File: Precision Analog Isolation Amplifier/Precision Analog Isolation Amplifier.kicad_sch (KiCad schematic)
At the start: 20 parts, among them J1 Conn_Coaxial, J2 Conn_Coaxial, Q1 2N3906, U1 HCNR201, U2 TLV172IDCK, U3 TLV172IDCK

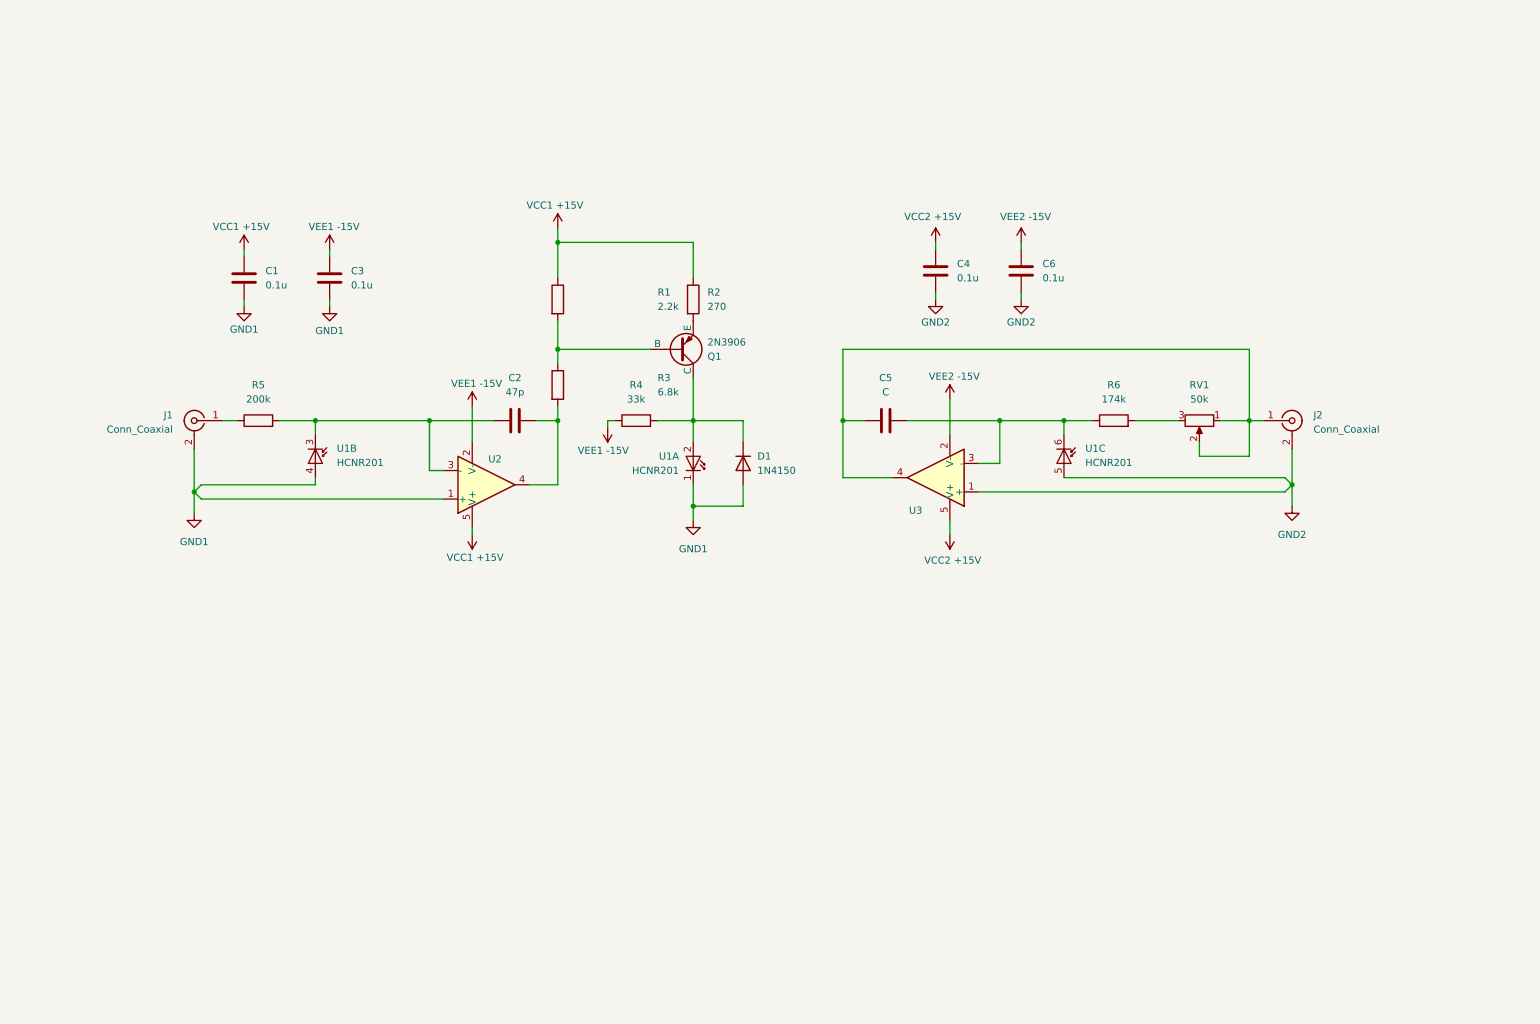
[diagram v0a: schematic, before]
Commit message: Add few components & Start PCB design
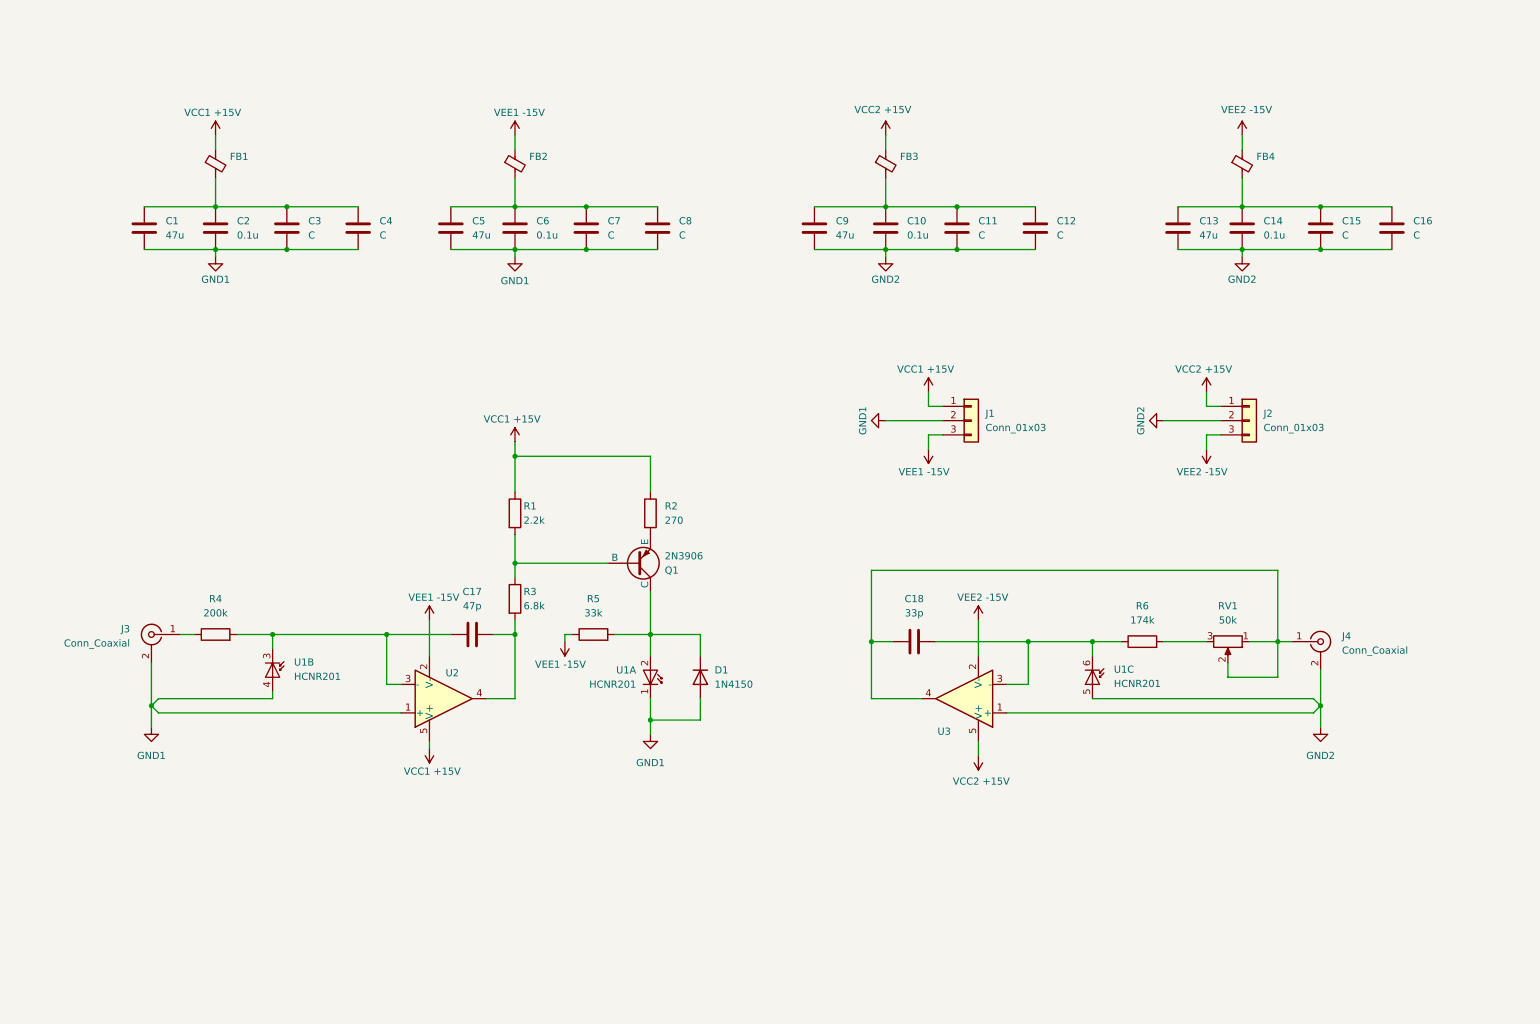
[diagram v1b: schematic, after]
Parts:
- added C1, C13, C5, C9: 47u, Capacitor_SMD:C_0805_2012Metric_Pad1.18x1.45mm_HandSolder, symbol Device:C
- added C11, C12, C15, C16, C3, C4, C7, C8: C, Capacitor_SMD:C_0805_2012Metric_Pad1.18x1.45mm_HandSolder, symbol Device:C
- added FB1, FB2, FB3, FB4: FerriteBead_Small, Inductor_SMD:L_1206_3216Metric, symbol Device:FerriteBead_Small
- added J1, J2: Conn_01x03, Connector_PinHeader_2.54mm:PinHeader_1x03_P2.54mm_Vertical, symbol Connector_Generic:Conn_01x03
- C10: renamed from C4; footprint (none) -> Capacitor_SMD:C_0805_2012Metric_Pad1.18x1.45mm_HandSolder
- C14: renamed from C6; footprint (none) -> Capacitor_SMD:C_0805_2012Metric_Pad1.18x1.45mm_HandSolder
- C17: renamed from C2; footprint (none) -> Capacitor_SMD:C_0805_2012Metric_Pad1.18x1.45mm_HandSolder
- C18: renamed from C5; value C -> 33p; footprint (none) -> Capacitor_SMD:C_0805_2012Metric_Pad1.18x1.45mm_HandSolder
- C2: renamed from C1; footprint (none) -> Capacitor_SMD:C_0805_2012Metric_Pad1.18x1.45mm_HandSolder
- C6: renamed from C3; footprint (none) -> Capacitor_SMD:C_0805_2012Metric_Pad1.18x1.45mm_HandSolder
- J3: renamed from J1; footprint (none) -> Connector_Coaxial:SMA_Amphenol_132289_EdgeMount
- J4: renamed from J2; footprint (none) -> Connector_Coaxial:SMA_Amphenol_132289_EdgeMount
- R1, R2, R3, R6: footprint (none) -> Resistor_SMD:R_0805_2012Metric_Pad1.20x1.40mm_HandSolder
- R4: renamed from R5; footprint (none) -> Resistor_SMD:R_0805_2012Metric_Pad1.20x1.40mm_HandSolder
- R5: renamed from R4; footprint (none) -> Resistor_SMD:R_0805_2012Metric_Pad1.20x1.40mm_HandSolder
- RV1: footprint (none) -> Potentiometer_THT:Potentiometer_Bourns_3386W_Horizontal
- U2, U3: footprint Package_TO_SOT_SMD:SOT-353_SC-70-5 -> (none)
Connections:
- net GND1: now also C1.1, C3.1, C4.1, C5.1, C7.1, C8.1, J1.2 (Pin_2)
- net GND2: now also C11.1, C12.1, C13.1, C15.1, C16.1, C9.1, J2.2 (Pin_2)
- net VCC1 +15V: now also FB1.1, J1.1 (Pin_1); no longer C2.2
- net VCC2 +15V: now also FB3.1, J2.1 (Pin_1); no longer C10.2
- net VEE1 -15V: now also FB2.1, J1.3 (Pin_3); no longer C6.2
- net VEE2 -15V: now also FB4.1, J2.3 (Pin_3); no longer C14.2
- new net: C1.2, C2.2, C3.2, C4.2, FB1.2
- new net: C13.2, C14.2, C15.2, C16.2, FB4.2
- new net: C5.2, C6.2, C7.2, C8.2, FB2.2
- new net: C10.2, C11.2, C12.2, C9.2, FB3.2
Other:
- moved on the sheet: C10, C14, C17, C18, C2, C6, D1, J3, J4, Q1, R1, R2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

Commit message: Update Schematic & PCB
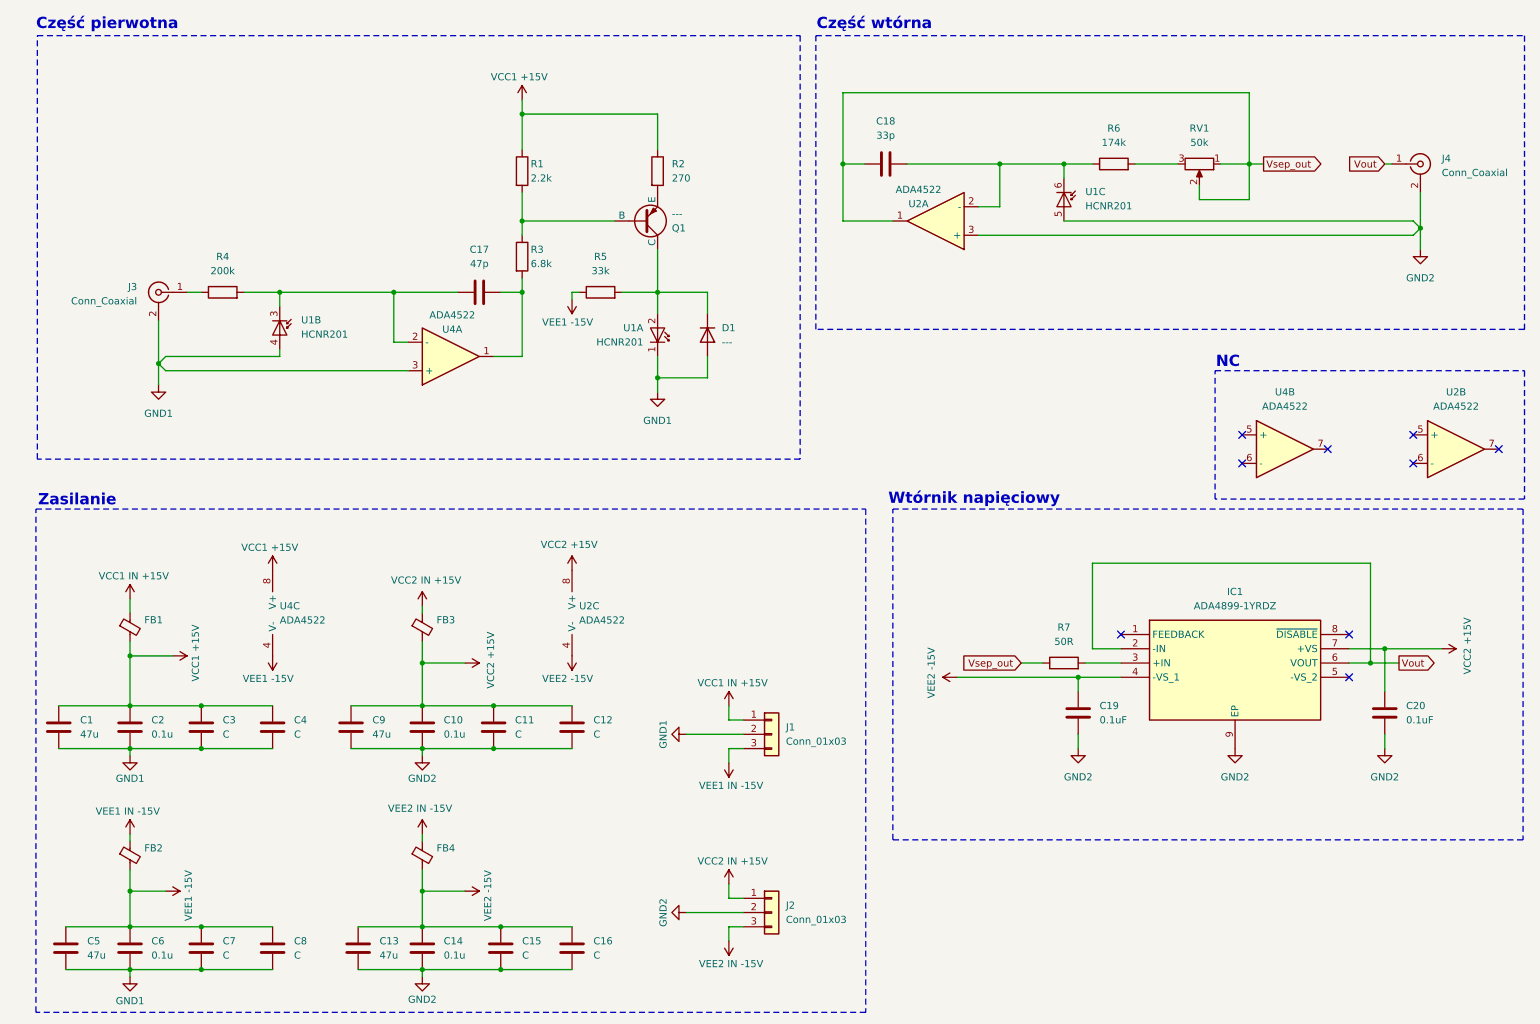
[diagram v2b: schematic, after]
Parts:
- removed U2, U3: TLV172IDCK, symbol Amplifier_Operational:TLV172IDCK
- added C19, C20: 0.1uF, Capacitor_SMD:C_0805_2012Metric_Pad1.18x1.45mm_HandSolder, symbol Device:C
- added IC1: ADA4899-1YRDZ, SOIC127P600X175-9N, symbol ADA4899:ADA4899-1YRDZ
- added R7: 50R, Resistor_SMD:R_0805_2012Metric_Pad1.20x1.40mm_HandSolder, symbol Device:R
- added U2, U4: ADA4522, ADA4522:SOIC127P600X175-8N, symbol Amplifier_Operational:OPA1692xDGK
- D1: value 1N4150 -> ---; footprint (none) -> Diode_SMD:D_0805_2012Metric_Pad1.15x1.40mm_HandSolder
- Q1: value 2N3906 -> ---; footprint (none) -> Package_TO_SOT_SMD:SOT-23_Handsoldering
- U1: footprint (none) -> HCNR201-300E:HCNR201300E
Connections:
- net GND1: now also U4.3 (+)
- net GND2: now also C19.1, C20.1, IC1.9 (EP), U2.3 (+)
- net VCC1 +15V: now also C1.2, C2.2, C3.2, C4.2, FB1.2, U4.8 (V+); no longer FB1.1, J1.1 (Pin_1)
- net VCC2 +15V: now also C10.2, C11.2, C12.2, C9.2, FB3.2, C20.2, IC1.7 (+VS), U2.8 (V+); no longer FB3.1, J2.1 (Pin_1)
- net VEE1 -15V: now also C5.2, C6.2, C7.2, C8.2, FB2.2, U4.4 (V-); no longer FB2.1, J1.3 (Pin_3)
- net VEE2 -15V: now also C13.2, C14.2, C15.2, C16.2, FB4.2, C19.2, IC1.4 (-VS_1), U2.4 (V-); no longer FB4.1, J2.3 (Pin_3)
- net at C17.1, R4.2, U1.3 (K): now also U4.2 (-)
- net at C17.2, R3.2: now also U4.1
- net at C18.2, R6.1, U1.6 (K): now also U2.2 (-)
- net Vsep_out: now reaches C18.1, RV1.1, RV1.2
- net Vsep_out: now also R7.1, U2.1; no longer J4.1 (In)
- new net: IC1.3 (+IN), R7.2
- new net VCC1 IN +15V: FB1.1, J1.1 (Pin_1)
- new net VCC2 IN +15V: FB3.1, J2.1 (Pin_1)
- new net VEE1 IN -15V: FB2.1, J1.3 (Pin_3)
- new net VEE2 IN -15V: FB4.1, J2.3 (Pin_3)
- new net Vout: IC1.2 (-IN), IC1.6 (VOUT), J4.1 (In)
- no-connect marks 0 -> 9
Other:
- note added: "Część pierwotna"
- note added: "Część wtórna"
- note added: "NC"
- note added: "Wtórnik napięciowy"
- note added: "Zasilanie"
- moved on the sheet: C1, C10, C11, C12, C13, C14, C15, C16, C17, C18, C2, C3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
